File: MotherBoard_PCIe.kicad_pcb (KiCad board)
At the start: 2 copper layers, 100 x 100 mm, 27 parts, among them J1 Conn_01x04, J2 Conn_01x07, J3 Conn_01x04, J4 Conn_01x07, J5 Bus_PCIexpress_x16_164_Positi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, J6 Bus_PCIexpress_x16_164_Positi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, J7 Bus_PCIexpress_x16_164_Positi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

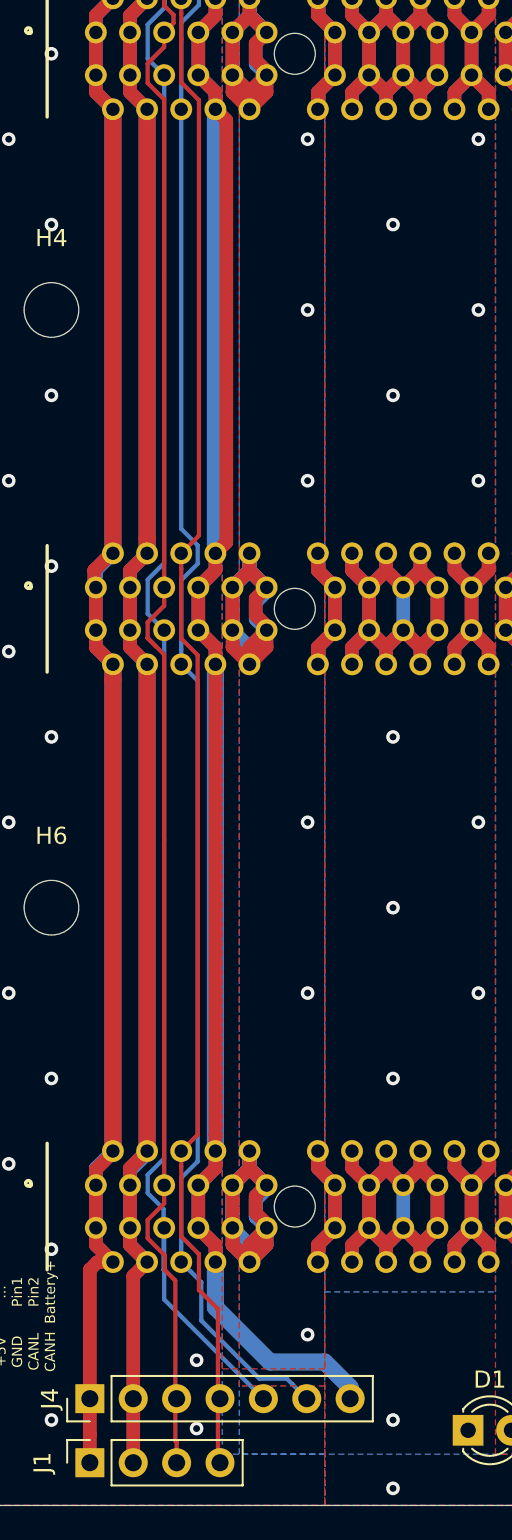
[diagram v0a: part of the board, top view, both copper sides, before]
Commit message: +Battery Strong
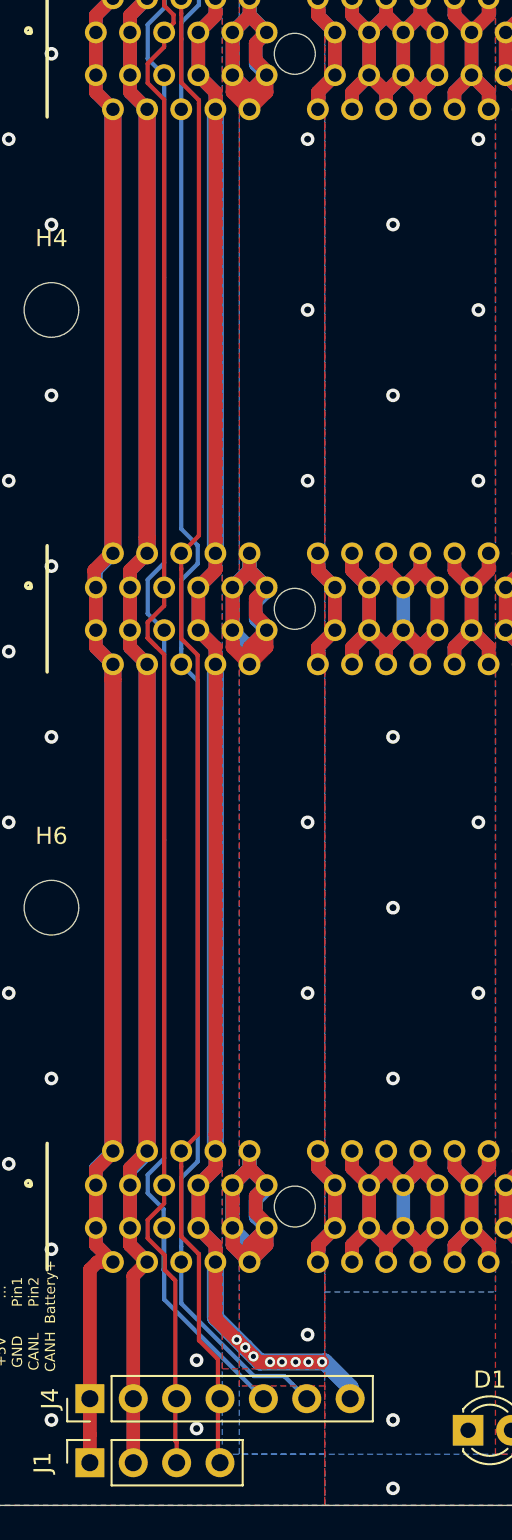
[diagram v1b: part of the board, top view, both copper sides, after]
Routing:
- net +BATT: track 176.3 -> 186.7 mm, vias 0 -> 8
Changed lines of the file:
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@@
     (thickness 1.6)
     (drawings 14)
-    (tracks 2031)
+    (tracks 2047)
     (zones 0)
     (modules 27)
@@
     (0 F.Cu signal)
     (31 B.Cu signal)
-    (32 B.Adhes user)
-    (33 F.Adhes user)
-    (34 B.Paste user)
-    (35 F.Paste user)
-    (36 B.SilkS user)
-    (37 F.SilkS user)
-    (38 B.Mask user)
-    (39 F.Mask user)
-    (40 Dwgs.User user)
-    (41 Cmts.User user)
-    (42 Eco1.User user)
-    (43 Eco2.User user)
-    (44 Edge.Cuts user)
-    (45 Margin user)
-    (46 B.CrtYd user)
-    (47 F.CrtYd user)
-    (48 B.Fab user)
-    (49 F.Fab user)
+    (32 B.Adhes user hide)
+    (33 F.Adhes user hide)
+    (34 B.Paste user hide)
+    (35 F.Paste user hide)
+    (36 B.SilkS user hide)
+    (37 F.SilkS user hide)
+    (38 B.Mask user hide)
+    (39 F.Mask user hide)
+    (40 Dwgs.User user hide)
+    (41 Cmts.User user hide)
+    (42 Eco1.User user hide)
+    (43 Eco2.User user hide)
+    (44 Edge.Cuts user hide)
+    (45 Margin user hide)
+    (46 B.CrtYd user hide)
+    (47 F.CrtYd user hide)
+    (48 B.Fab user hide)
+    (49 F.Fab user hide)
   )
   (setup
-    (last_trace_width 0.25)
+    (last_trace_width 0.8)
     (user_trace_width 0.2)
     (user_trace_width 0.4)
@@
   (via (at 170 52) (size 0.8) (drill 0.4) (layers F.Cu B.Cu) (net 2))
   (segment (start 114.6 94.25) (end 114.6 68.25) (width 1) (layer B.Cu) (net 3))
-  (segment (start 115.239999 93.610001) (end 115.239999 68.889999) (width 0.8) (layer F.Cu) (net 3))
-  (segment (start 114.6 94.25) (end 115.239999 93.610001) (width 0.8) (layer F.Cu) (net 3))
   (segment (start 114.6 128.275318) (end 114.6 129.25) (width 0.8) (layer F.Cu) (net 3))
   (segment (start 114.6 100.75) (end 114.6 128.275318) (width 0.8) (layer F.Cu) (net 3))
-  (segment (start 115.239999 68.889999) (end 114.6 68.25) (width 0.8) (layer F.Cu) (net 3))
   (segment (start 114.6 95.25) (end 113.6 96.25) (width 0.8) (layer F.Cu) (net 3))
   (segment (start 114.6 94.25) (end 114.6 95.25) (width 0.8) (layer F.Cu) (net 3))
@@
   (segment (start 114.6 100.75) (end 114.6 99.75) (width 0.8) (layer B.Cu) (net 3))
   (segment (start 114.6 129.25) (end 114.6 101.25) (width 1) (layer B.Cu) (net 3))
-  (segment (start 114.6 138.4) (end 117.8 141.6) (width 1) (layer B.Cu) (net 3))
-  (segment (start 114.6 135.75) (end 114.6 138.4) (width 1) (layer B.Cu) (net 3))
-  (segment (start 117.8 141.6) (end 121 141.6) (width 1) (layer B.Cu) (net 3))
-  (segment (start 121 141.6) (end 122.49 143.09) (width 1) (layer B.Cu) (net 3))
+  (segment (start 114.6 94.25) (end 114.6 68.25) (width 0.8) (layer F.Cu) (net 3))
   (segment (start 122.49 143.09) (end 122.49 143.75) (width 1) (layer B.Cu) (net 3))
+  (segment (start 121 141.6) (end 122.49 143.09) (width 1) (layer B.Cu) (net 3))
+  (segment (start 117.2 141.6) (end 121 141.6) (width 1) (layer B.Cu) (net 3))
+  (segment (start 114.6 139) (end 116.35 140.75) (width 1) (layer B.Cu) (net 3))
+  (segment (start 114.6 135.75) (end 114.6 139) (width 1) (layer B.Cu) (net 3))
+  (segment (start 114.6 135.75) (end 114.6 139.05) (width 0.8) (layer F.Cu) (net 3))
+  (segment (start 114.6 139.05) (end 115.85 140.3) (width 0.8) (layer F.Cu) (net 3))
+  (segment (start 117.15 141.6) (end 117.8 141.6) (width 0.8) (layer F.Cu) (net 3))
+  (segment (start 120.85 141.6) (end 120.85 141.6) (width 0.8) (layer F.Cu) (net 3))
+  (via (at 120.85 141.6) (size 0.6) (drill 0.3) (layers F.Cu B.Cu) (net 3))
+  (segment (start 120.05 141.6) (end 120.85 141.6) (width 0.8) (layer F.Cu) (net 3))
+  (via (at 120.05 141.6) (size 0.6) (drill 0.3) (layers F.Cu B.Cu) (net 3))
+  (segment (start 119.3 141.6) (end 120.05 141.6) (width 0.8) (layer F.Cu) (net 3))
+  (via (at 119.3 141.6) (size 0.6) (drill 0.3) (layers F.Cu B.Cu) (net 3))
+  (segment (start 118.5 141.6) (end 119.3 141.6) (width 0.8) (layer F.Cu) (net 3))
+  (via (at 118.5 141.6) (size 0.6) (drill 0.3) (layers F.Cu B.Cu) (net 3))
+  (segment (start 117.8 141.6) (end 118.5 141.6) (width 0.8) (layer F.Cu) (net 3))
+  (via (at 117.8 141.6) (size 0.6) (drill 0.3) (layers F.Cu B.Cu) (net 3))
+  (segment (start 116.825 141.275) (end 117.15 141.6) (width 0.8) (layer F.Cu) (net 3))
+  (via (at 116.825 141.275) (size 0.6) (drill 0.3) (layers F.Cu B.Cu) (net 3))
+  (segment (start 116.35 140.75) (end 117.2 141.6) (width 1) (layer B.Cu) (net 3))
+  (via (at 116.35 140.75) (size 0.6) (drill 0.3) (layers F.Cu B.Cu) (net 3))
+  (segment (start 115.85 140.3) (end 116.825 141.275) (width 0.8) (layer F.Cu) (net 3))
+  (via (at 115.85 140.3) (size 0.6) (drill 0.3) (layers F.Cu B.Cu) (net 3))
   (segment (start 112.6 99.844904) (end 112.6 100.75) (width 0.25) (layer B.Cu) (net 4))
   (segment (start 112.6 95.821798) (end 112.6 99.844904) (width 0.25) (layer B.Cu) (net 4))
@@
   (segment (start 112.6 63.178202) (end 113.634999 62.143203) (width 0.25) (layer B.Cu) (net 4))
   (segment (start 112.6 68.25) (end 112.6 63.178202) (width 0.25) (layer B.Cu) (net 4))
-  (segment (start 112.6 135.75) (end 113.77499 136.92499) (width 0.25) (layer B.Cu) (net 4))
+  (segment (start 116.85827 142.425011) (end 118.625011 142.425011) (width 0.25) (layer B.Cu) (net 4))
+  (segment (start 118.625011 142.425011) (end 119.100001 142.900001) (width 0.25) (layer B.Cu) (net 4))
+  (segment (start 112.6 135.75) (end 112.6 138.166741) (width 0.25) (layer B.Cu) (net 4))
+  (segment (start 112.6 138.166741) (end 116.85827 142.425011) (width 0.25) (layer B.Cu) (net 4))
   (segment (start 119.100001 142.900001) (end 119.95 143.75) (width 0.25) (layer B.Cu) (net 4))
-  (segment (start 113.77499 136.92499) (end 113.77499 139.17499) (width 0.25) (layer B.Cu) (net 4))
-  (segment (start 117.174999 142.574999) (end 118.774999 142.574999) (width 0.25) (layer B.Cu) (net 4))
-  (segment (start 113.77499 139.17499) (end 117.174999 142.574999) (width 0.25) (layer B.Cu) (net 4))
-  (segment (start 118.774999 142.574999) (end 119.100001 142.900001) (width 0.25) (layer B.Cu) (net 4))
   (segment (start 111.6 133.75) (end 111.6 136.178202) (width 0.25) (layer B.Cu) (net 5))
   (segment (start 113.26 60.4) (end 117.41 56.25) (width 0.25) (layer B.Cu) (net 5))
@@
   (segment (start 113.634999 67.889101) (end 113.634999 67.713201) (width 0.25) (layer F.Cu) (net 9))
   (segment (start 113.634999 67.713201) (end 112.6 66.678202) (width 0.25) (layer F.Cu) (net 9))
+  (segment (start 114.8 59.55) (end 112.6 61.75) (width 0.25) (layer F.Cu) (net 9))
+  (segment (start 114.87 52.5) (end 114.8 52.57) (width 0.25) (layer F.Cu) (net 9))
+  (segment (start 114.8 52.57) (end 114.8 59.55) (width 0.25) (layer F.Cu) (net 9))
   (segment (start 112.6 130.155096) (end 112.6 129.25) (width 0.25) (layer F.Cu) (net 9))
-  (segment (start 114.75 147.38) (end 114.75 138.5) (width 0.25) (layer F.Cu) (net 9))
+  (segment (start 112.6 134.2482) (end 112.6 130.155096) (width 0.25) (layer F.Cu) (net 9))
   (segment (start 114.87 147.5) (end 114.75 147.38) (width 0.25) (layer F.Cu) (net 9))
-  (segment (start 114.75 138.5) (end 113.634999 137.384999) (width 0.25) (layer F.Cu) (net 9))
-  (segment (start 113.634999 137.384999) (end 113.634999 135.286799) (width 0.25) (layer F.Cu) (net 9))
+  (segment (start 114.75 147.38) (end 114.75 141.45) (width 0.25) (layer F.Cu) (net 9))
+  (segment (start 113.634999 140.334999) (end 113.634999 135.286799) (width 0.25) (layer F.Cu) (net 9))
   (segment (start 113.634999 135.286799) (end 113.636799 135.284999) (width 0.25) (layer F.Cu) (net 9))
-  (segment (start 112.6 134.2482) (end 112.6 130.155096) (width 0.25) (layer F.Cu) (net 9))
+  (segment (start 114.75 141.45) (end 113.634999 140.334999) (width 0.25) (layer F.Cu) (net 9))
   (segment (start 113.636799 135.284999) (end 112.6 134.2482) (width 0.25) (layer F.Cu) (net 9))
-  (segment (start 114.8 59.55) (end 112.6 61.75) (width 0.25) (layer F.Cu) (net 9))
-  (segment (start 114.87 52.5) (end 114.8 52.57) (width 0.25) (layer F.Cu) (net 9))
-  (segment (start 114.8 52.57) (end 114.8 59.55) (width 0.25) (layer F.Cu) (net 9))
   (segment (start 132.04 145.5) (end 135.092082 145.5) (width 0.6) (layer F.Cu) (net 10))
   (zone (net 2) (net_name GNDPWR) (layer F.Cu) (hatch edge 0.508)

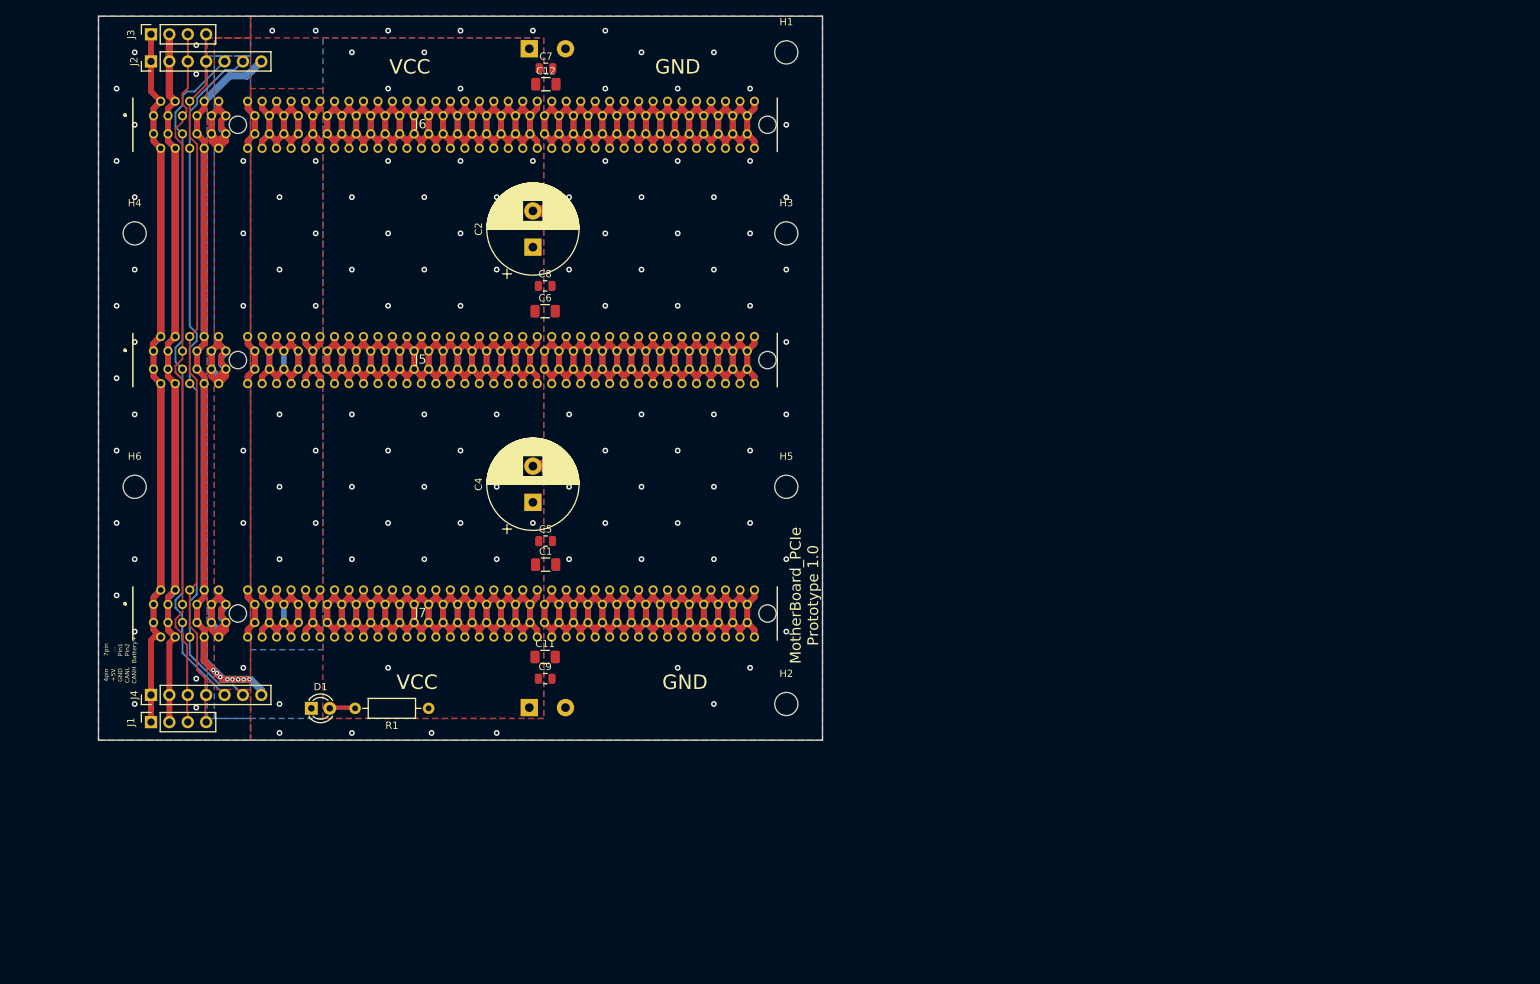
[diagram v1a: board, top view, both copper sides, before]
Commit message: buck-up
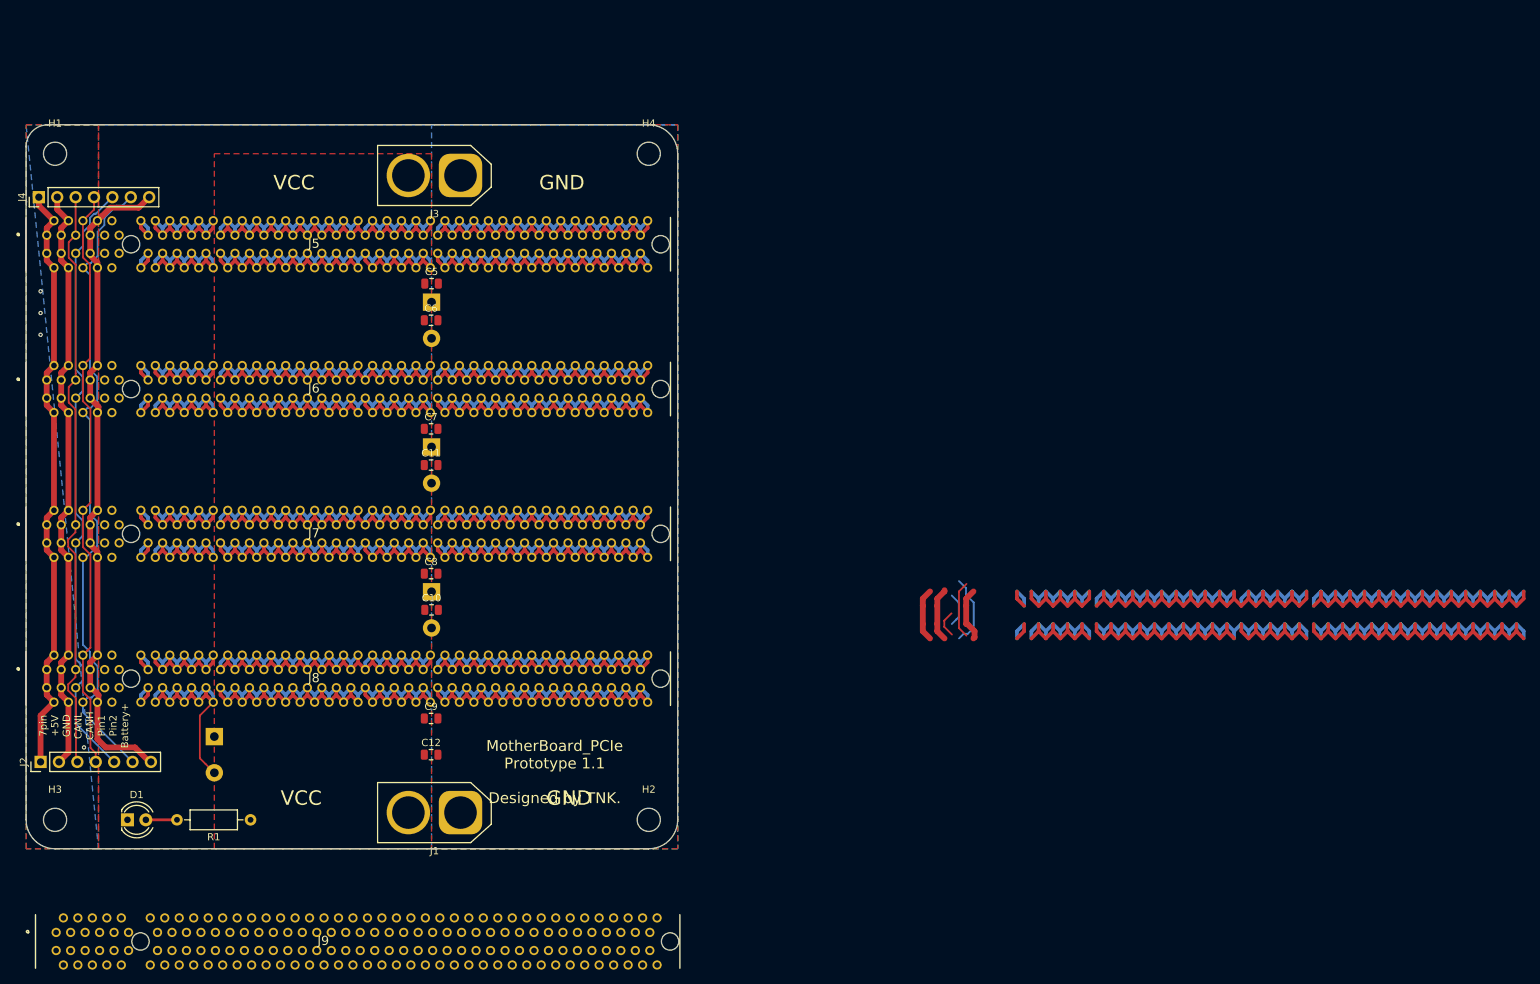
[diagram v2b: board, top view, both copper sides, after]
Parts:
- removed H5, H6: MountingHole, MountingHole:MountingHole_3.2mm_M3
- added J8: Bus_PCIexpress_x16_164_Position, SamacSys_Parts:10018783-10113TLF, F.Cu at (90.0, 141.5)
- added J9: Bus_mechaken_PCIexpress_x16_164_Position, PCIe:Socket_mechaken_PCIexpress_x16_164_position, F.Cu at (91.3, 177.8)
- C1: value 10uF -> 1000uF; footprint Capacitor_SMD:C_1206_3216Metric -> Capacitor_THT:CP_Radial_D12.5mm_P5.00mm; moved to B.Cu
- C10: value 1000uF -> 10uF; footprint Capacitor_THT:CP_Radial_D12.5mm_P5.00mm -> Capacitor_SMD:C_0805_2012Metric; moved to F.Cu
- C11, C12, C6: footprint Capacitor_SMD:C_1206_3216Metric -> Capacitor_SMD:C_0805_2012Metric
- C2, C4: moved to B.Cu
- C5, C7, C8, C9: value 0.1uF -> 1uF
- D1: footprint LED_THT:LED_D3.0mm -> LED_THT:LED_D4.0mm
- J1: value Conn_01x04 -> Conn_01x02; footprint Connector_PinSocket_2.54mm:PinSocket_1x04_P2.54mm_Vertical -> Connector_AMASS:AMASS_XT60-F_1x02_P7.20mm_Vertical
- J3: value Conn_01x04 -> Conn_01x02; footprint Connector_PinSocket_2.54mm:PinSocket_1x04_P2.54mm_Vertical -> Connector_AMASS:AMASS_XT60-M_1x02_P7.20mm_Vertical
- moved H3 129.5 mm to (94.0, 161.0)
- moved H1 102.0 mm to (94.0, 69.0)
- moved J2 97.9 mm to (92.0, 153.0)
- moved C12 93.9 mm to (145.9, 152.0)
- moved H4 71.8 mm to (176.0, 69.0)
- moved J4 70.5 mm to (91.8, 75.0)
- moved C4 54.6 mm to (116.0, 149.5), turned to 270 degrees
- moved C7 52.3 mm to (145.9, 107.0)
- moved J3 47.0 mm to (150.0, 72.0), turned to 180 degrees
- moved J1 44.5 mm to (150.0, 160.0), turned to 180 degrees
- moved C8 42.8 mm to (145.9, 127.0)
- moved J6 39.4 mm to (90.0, 101.5)
- moved C5 38.9 mm to (146.0, 86.9)
- moved C3 37.5 mm to (146.0, 89.5), turned to 270 degrees
- moved C2 30.9 mm to (146.0, 109.5), turned to 270 degrees
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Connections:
- J1 pad 1: +5V -> GNDPWR
- J1 pad 2: GND -> VCC
- J3 pad 1: +5V -> GNDPWR
- J3 pad 2: GND -> VCC
- J5 pad B5: Pin_B4 -> Pin_B5
- J5 pad B6: Pin_B5 -> Pin_B6
- J6 pad B5: Pin_B4 -> Pin_B5
- J6 pad B6: Pin_B5 -> Pin_B6
- J7 pad B5: Pin_B4 -> Pin_B5
- J7 pad B6: Pin_B5 -> Pin_B6
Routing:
- net (no net): track 0.00 -> 567.0 mm
- net VCC: track 1121.2 -> 923.5 mm, vias 39 -> 0
- net GND: track 182.1 -> 82.5 mm, vias 20 -> 4
- net +BATT: track 186.7 -> 92.4 mm, vias 8 -> 0
- net +5V: track 175.5 -> 82.9 mm
- net GNDPWR: track 1217.4 -> 1160.6 mm, vias 65 -> 0
- net CANL: track 99.2 -> 81.4 mm
- net CANH: track 98.6 -> 81.9 mm
- net Pin_B4: track 97.8 -> 84.8 mm
- net Pin_B5: track 97.0 -> 90.1 mm
- net Net-(D1-Pad2): track 3.05 -> 4.30 mm
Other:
- board size 100 x 100 mm -> 90 x 100 mm
- board text added: "7pin +5V GND CANL CANH Pin1 Pin2 Battery+"
- board text added: "MotherBoard_PCIe Prototype 1.1"
- board text removed: "4pin +5V GND CANL CANH"
- board text removed: "7pin ... Pin1 Pin2 Battery+"
- board text removed: "MotherBoard_PCIe Prototype 1.0"
